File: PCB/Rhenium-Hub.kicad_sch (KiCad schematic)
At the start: 23 parts, among them J1 USB_A, J2 USB_A, J3 USB_C_Receptacle_USB2.0_16P, J4 USB_C_Receptacle_USB2.0_16P, J5 USB_C_Receptacle_USB2.0_16P, U1 USB2514B_Bi

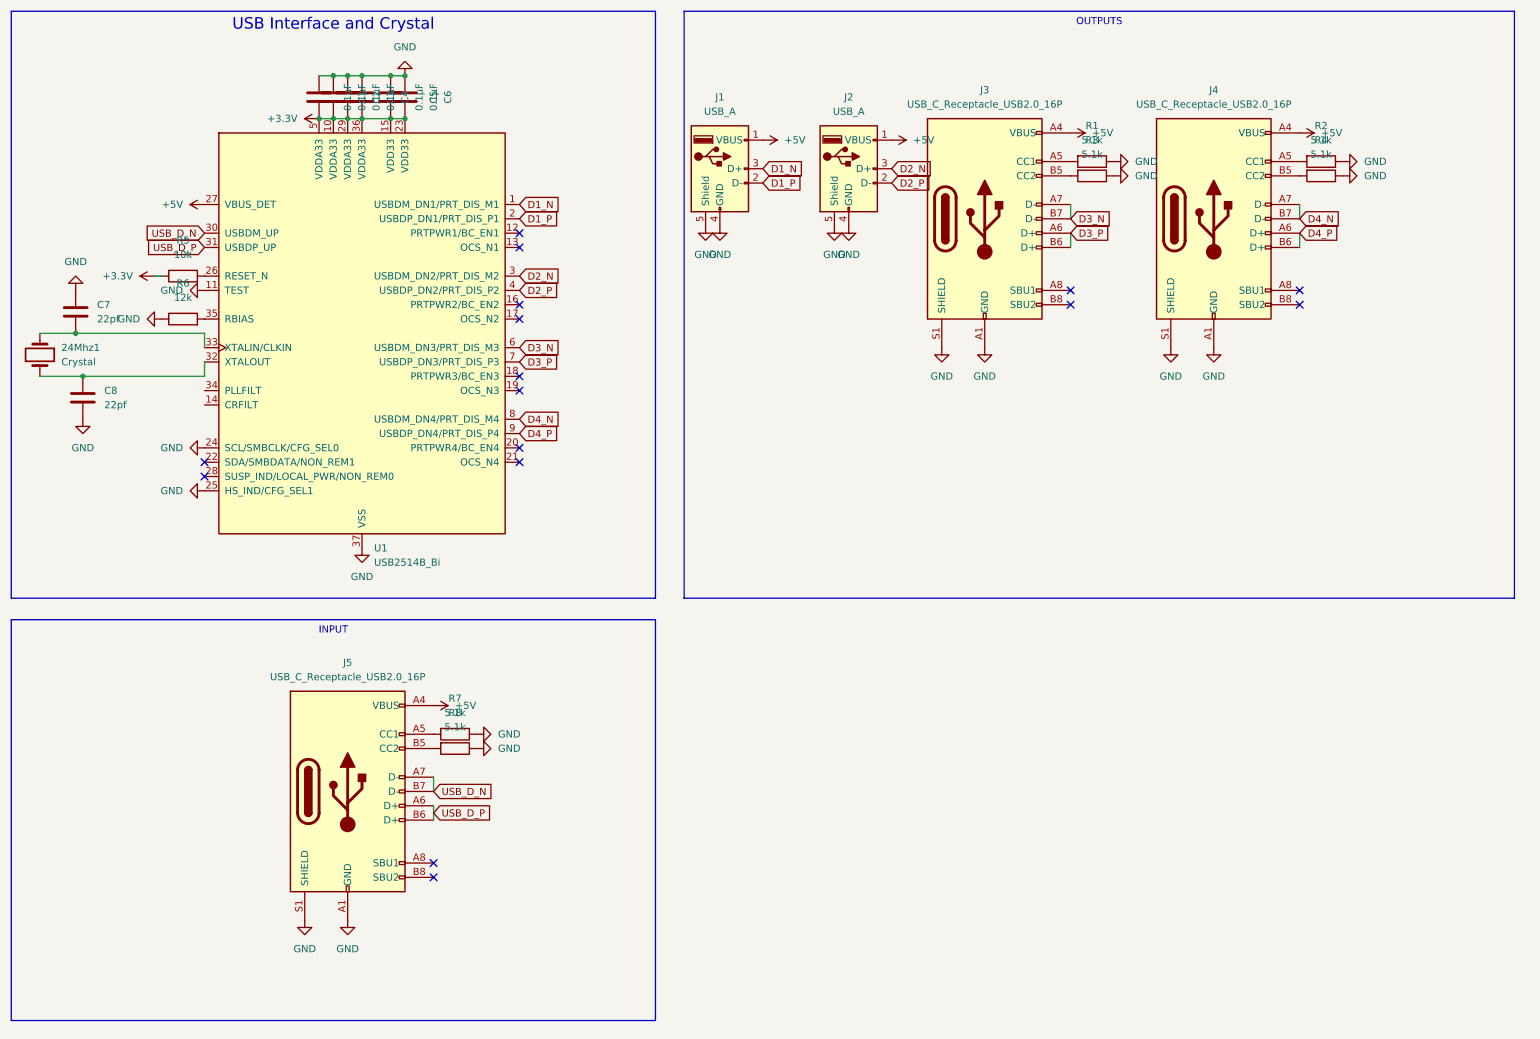
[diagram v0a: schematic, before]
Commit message: Updated the pcb
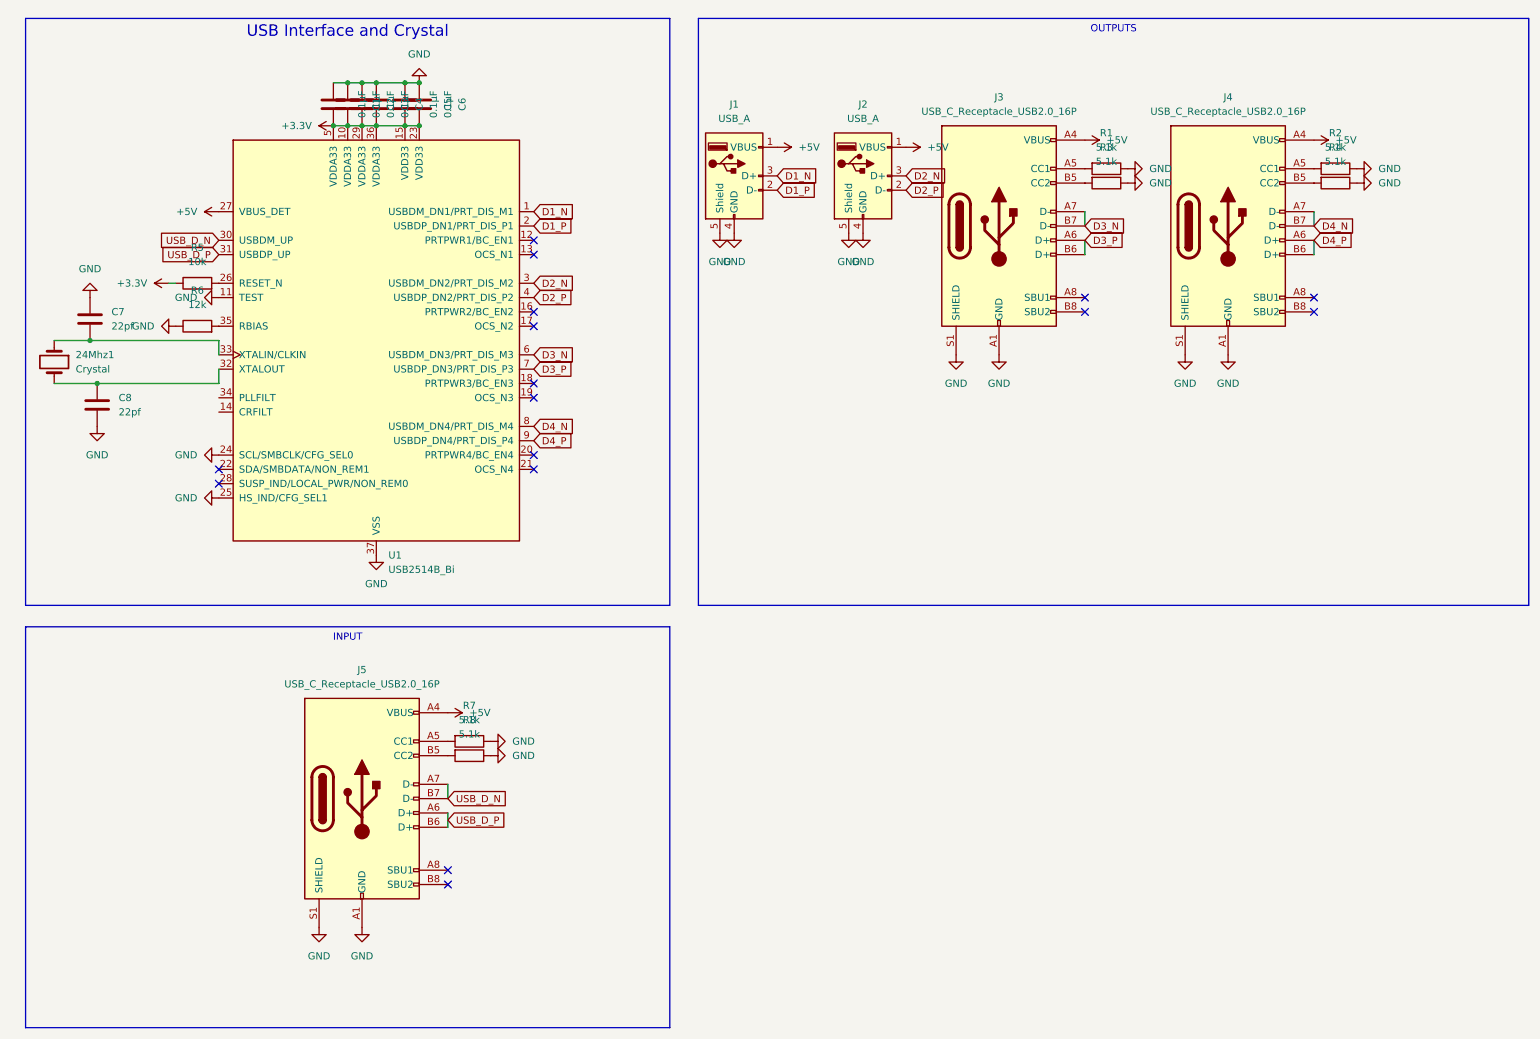
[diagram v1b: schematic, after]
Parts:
- J1, J2: footprint Connector_USB:USB_A_CNCTech_1001-011-01101_Horizontal -> Connector_USB:USB_A_Wuerth_614004134726_Horizontal
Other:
- moved on the sheet: 24Mhz1, C1, C2, C3, C4, C5, C6, C7, C8, J1, J2, J3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
